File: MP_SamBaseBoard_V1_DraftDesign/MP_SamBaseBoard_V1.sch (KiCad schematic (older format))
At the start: 36 parts, among them Q1 DMP3098L, U1 ESP32-WROOM-32, U2 ATSAMD51J19A-A, U3 74LVC1G125, U4 TPS62135, U5 TPS62086, Y1 Crystal

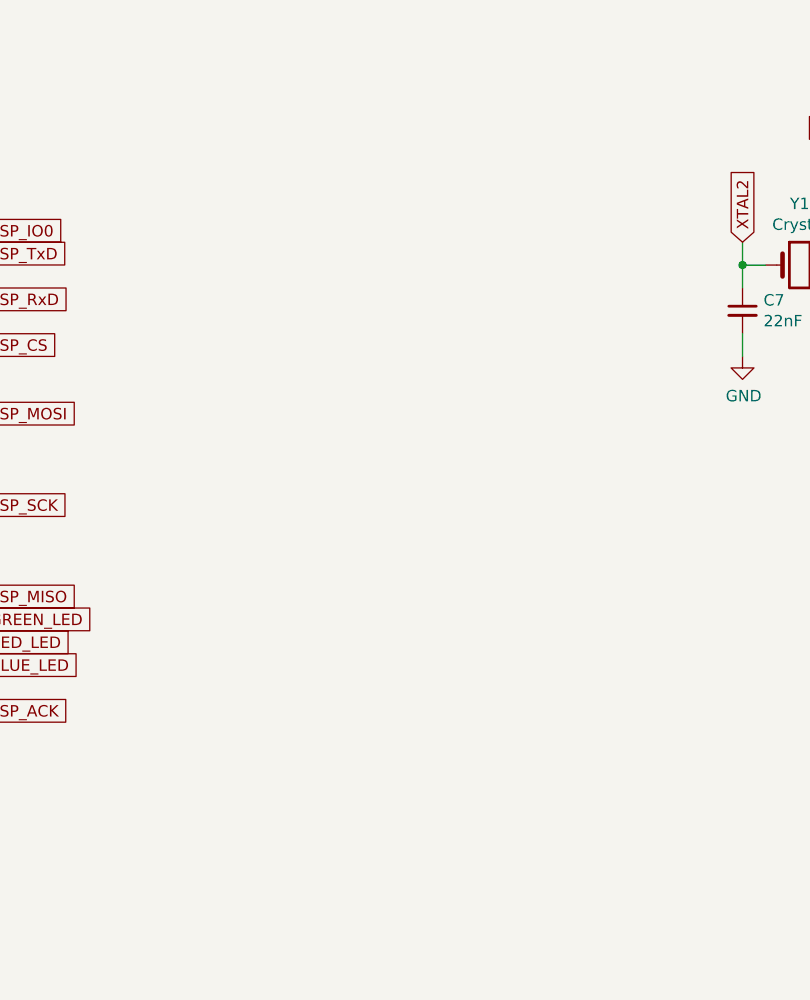
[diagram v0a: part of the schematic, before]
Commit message: update
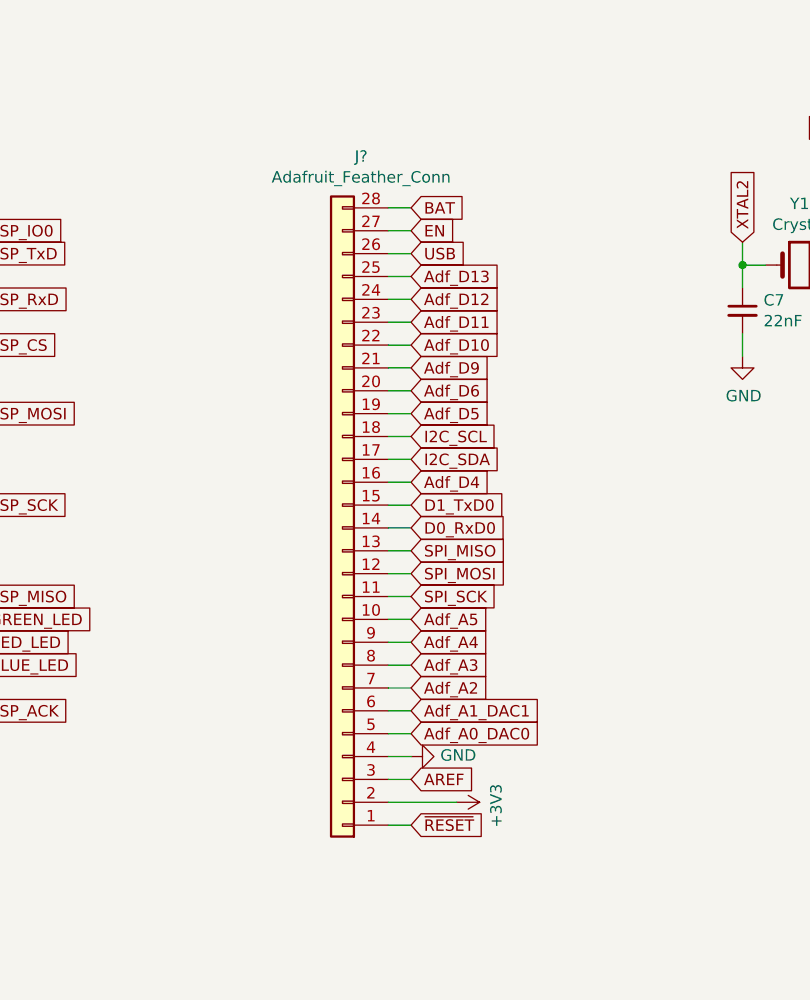
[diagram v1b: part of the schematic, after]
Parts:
- added J?: Adafruit_Feather_Conn, GiraffeTech-Connector:Adafruit-Feather_WoMountPoint, symbol Connector_Generic:Conn_01x28
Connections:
- net +3V3: now also J?.2 (Pin_2)
- net AREF: now also J?.3 (Pin_3)
- net Adf_A0_DAC0: now also J?.5 (Pin_5)
- net Adf_A1_DAC1: now also J?.6 (Pin_6)
- net Adf_A2: now also J?.7 (Pin_7)
- net Adf_A3: now also J?.8 (Pin_8)
- net Adf_A4: now also J?.9 (Pin_9)
- net Adf_A5: now also J?.10 (Pin_10)
- net Adf_D10: now also J?.22 (Pin_22)
- net Adf_D11: now also J?.23 (Pin_23)
- net Adf_D12: now also J?.24 (Pin_24)
- net Adf_D13: now also J?.25 (Pin_25)
- net Adf_D4: now also J?.16 (Pin_16)
- net Adf_D5: now also J?.19 (Pin_19)
- net Adf_D6: now also J?.20 (Pin_20)
- net Adf_D9: now also J?.21 (Pin_21)
- net D0_RxD0: now also J?.14 (Pin_14)
- net D1_TxD0: now also J?.15 (Pin_15)
- net GND: now also J?.4 (Pin_4)
- net I2C_SCL: now also J?.18 (Pin_18)
- net I2C_SDA: now also J?.17 (Pin_17)
- net SPI_MISO: now also J?.13 (Pin_13)
- net SPI_MOSI: now also J?.12 (Pin_12)
- net SPI_SCK: now also J?.11 (Pin_11)
- net ~RESET: now also J?.1 (Pin_1)
- new net BAT: J?.28 (Pin_28)
- new net EN: J?.27 (Pin_27)
- new net USB: J?.26 (Pin_26)
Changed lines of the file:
@@
 Wire Wire Line
 	12700 5300 12700 5400
+$Comp
+L Connector_Generic:Conn_01x28 J?
+U 1 1 5EB09696
+P 4800 2800
+F 0 "J?" H 4718 1175 50  0000 C CNN
+F 1 "Adafruit_Feather_Conn" H 4718 1266 50  0000 C CNN
+F 2 "GiraffeTech-Connector:Adafruit-Feather_WoMountPoint" H 4800 2800 50  0001 C CNN
+F 3 "~" H 4800 2800 50  0001 C CNN
+	1    4800 2800
+	-1   0    0    1
+$EndComp
+Wire Wire Line
+	5100 1400 5000 1400
+Wire Wire Line
+	5100 1500 5000 1500
+Wire Wire Line
+	5100 1600 5000 1600
+Wire Wire Line
+	5100 1700 5000 1700
+Wire Wire Line
+	5100 1800 5000 1800
+Wire Wire Line
+	5100 1900 5000 1900
+Wire Wire Line
+	5100 2000 5000 2000
+Wire Wire Line
+	5100 2100 5000 2100
+Wire Wire Line
+	5100 2200 5000 2200
+Wire Wire Line
+	5100 2300 5000 2300
+Wire Wire Line
+	5100 2400 5000 2400
+Wire Wire Line
+	5100 2500 5000 2500
+Wire Wire Line
+	5100 2600 5000 2600
+Wire Wire Line
+	5100 2700 5000 2700
+Wire Wire Line
+	5100 2800 5000 2800
+Wire Wire Line
+	5100 2900 5000 2900
+Wire Wire Line
+	5100 3000 5000 3000
+Wire Wire Line
+	5100 3100 5000 3100
+Wire Wire Line
+	5100 3200 5000 3200
+Wire Wire Line
+	5100 3300 5000 3300
+Wire Wire Line
+	5100 3400 5000 3400
+Wire Wire Line
+	5100 3500 5000 3500
+Wire Wire Line
+	5100 3600 5000 3600
+Wire Wire Line
+	5100 3700 5000 3700
+Wire Wire Line
+	5100 3800 5000 3800
+Wire Wire Line
+	5100 3900 5000 3900
+Wire Wire Line
+	5300 4000 5000 4000
+Wire Wire Line
+	5100 4100 5000 4100
+Text GLabel 5100 1400 2    50   Input ~ 0
+BAT
+Text GLabel 5100 1500 2    50   Input ~ 0
+EN
+Text GLabel 5100 1600 2    50   Input ~ 0
+USB
+Text GLabel 5100 2800 2    50   Input ~ 0
+D0_RxD0
+Text GLabel 5100 2700 2    50   Input ~ 0
+D1_TxD0
+Text GLabel 5100 2100 2    50   Input ~ 0
+Adf_D9
+Text GLabel 5100 2000 2    50   Input ~ 0
+Adf_D10
+Text GLabel 5100 1900 2    50   Input ~ 0
+Adf_D11
+Text GLabel 5100 1800 2    50   Input ~ 0
+Adf_D12
+Text GLabel 5100 1700 2    50   Input ~ 0
+Adf_D13
+Text GLabel 5100 2300 2    50   Input ~ 0
+Adf_D5
+Text GLabel 5100 2200 2    50   Input ~ 0
+Adf_D6
+Text GLabel 5100 2500 2    50   Input ~ 0
+I2C_SDA
+Text GLabel 5100 2400 2    50   Input ~ 0
+I2C_SCL
+Text GLabel 5100 2600 2    50   Input ~ 0
+Adf_D4
+Text GLabel 5100 2900 2    50   Input ~ 0
+SPI_MISO
+Text GLabel 5100 3000 2    50   Input ~ 0
+SPI_MOSI
+Text GLabel 5100 3100 2    50   Input ~ 0
+SPI_SCK
+Text GLabel 5100 3300 2    50   Input ~ 0
+Adf_A4
+Text GLabel 5100 3200 2    50   Input ~ 0
+Adf_A5
+Text GLabel 5100 3700 2    50   Input ~ 0
+Adf_A0_DAC0
+Text GLabel 5100 3600 2    50   Input ~ 0
+Adf_A1_DAC1
+Text GLabel 5100 3500 2    50   Input ~ 0
+Adf_A2
+Text GLabel 5100 3400 2    50   Input ~ 0
+Adf_A3
+$Comp
+L power:GND #PWR?
+U 1 1 5EDE7447
+P 5100 3800
+F 0 "#PWR?" H 5100 3550 50  0001 C CNN
+F 1 "GND" V 5105 3672 50  0000 R CNN
+F 2 "" H 5100 3800 50  0001 C CNN
+F 3 "" H 5100 3800 50  0001 C CNN
+	1    5100 3800
+	0    -1   -1   0
+$EndComp
+Text GLabel 5100 3900 2    50   Input ~ 0
+AREF
+$Comp
+L power:+3V3 #PWR?
+U 1 1 5EDEC800
+P 5300 4000
+F 0 "#PWR?" H 5300 3850 50  0001 C CNN
+F 1 "+3V3" H 5315 4173 50  0000 C CNN
+F 2 "" H 5300 4000 50  0001 C CNN
+F 3 "" H 5300 4000 50  0001 C CNN
+	1    5300 4000
+	0    1    1    0
+$EndComp
+Text GLabel 5100 4100 2    50   Input ~ 0
+~RESET
 $EndSCHEMATC
